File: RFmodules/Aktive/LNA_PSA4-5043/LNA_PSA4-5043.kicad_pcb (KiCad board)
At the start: 2 copper layers, 18 x 7.6 mm, 7 parts, among them U1 PSA4-5043+

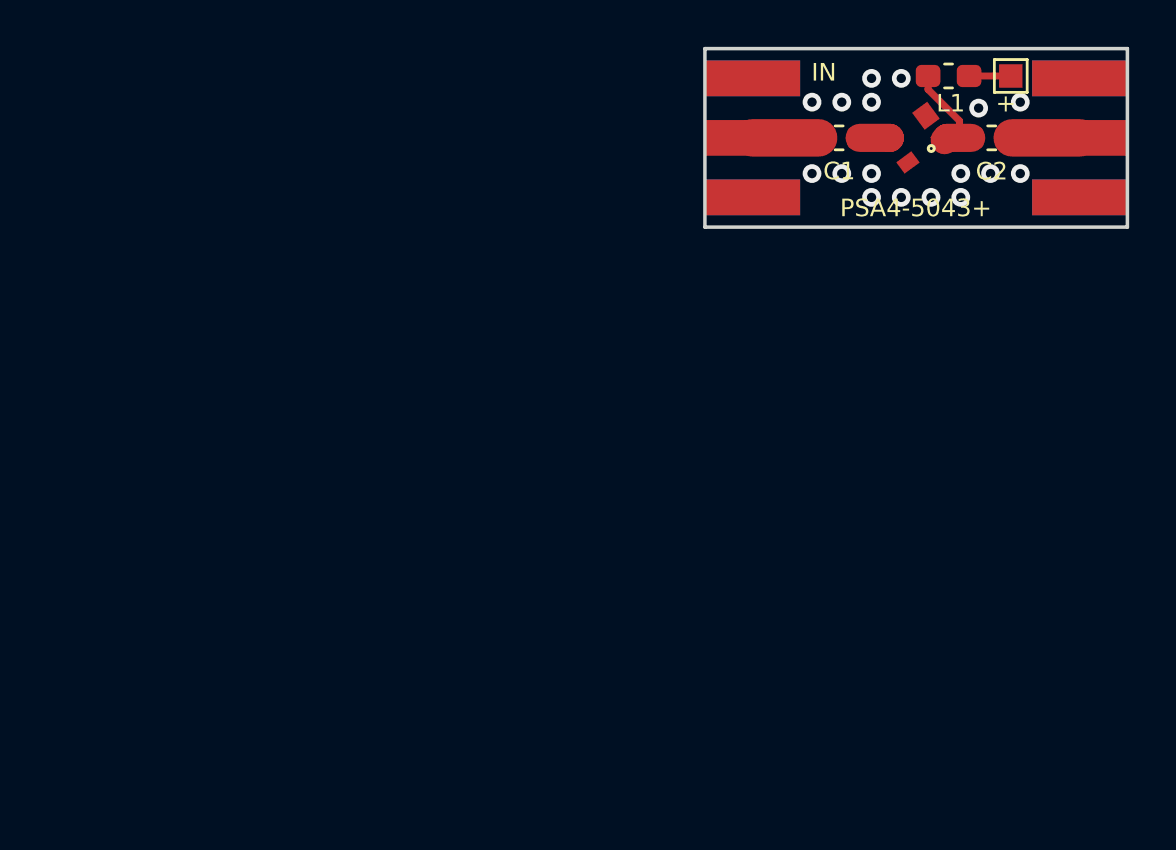
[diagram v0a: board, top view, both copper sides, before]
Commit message: Update LNA PSA4-5043 module to use new template
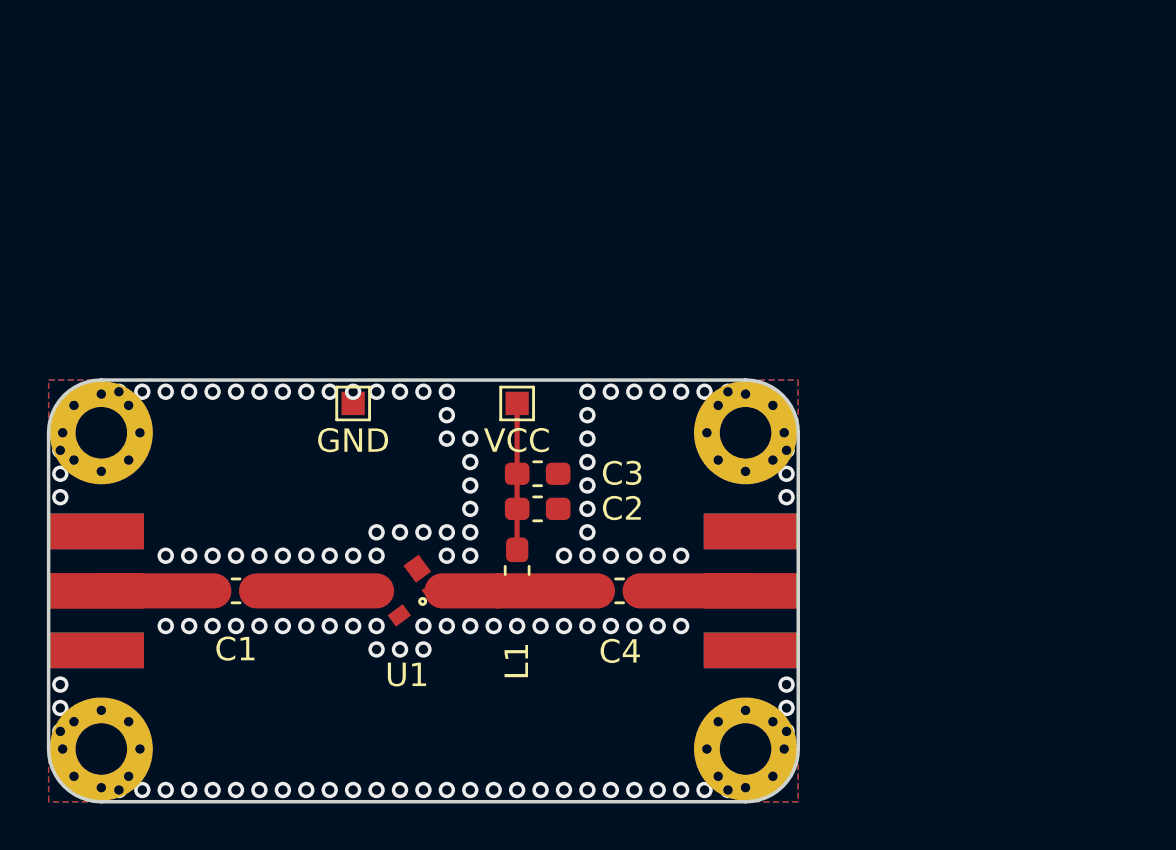
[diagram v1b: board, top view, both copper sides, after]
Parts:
- removed +: TestPoint, TestPoint:TestPoint_Pad_1.0x1.0mm
- removed IN, OUT: SMA, RFLego_Footprint:SMA_Edge
- added C3: C, Capacitor_SMD:C_0603_1608Metric_Pad1.05x0.95mm_HandSolder, F.Cu at (120.9, 104.0)
- added C4: C, Capacitor_SMD:C_0603_1608Metric_Pad1.05x0.95mm_HandSolder, F.Cu at (124.4, 109.0)
- added GND: GND, TestPoint:TestPoint_Pad_1.0x1.0mm, F.Cu at (113.0, 101.0)
- added H1: MountingHole_Pad, MountingHole:MountingHole_2.2mm_M2_Pad_Via, F.Cu at (102.2, 102.2)
- added H2: MountingHole_Pad, MountingHole:MountingHole_2.2mm_M2_Pad_Via, F.Cu at (102.2, 115.8)
- added H3: MountingHole_Pad, MountingHole:MountingHole_2.2mm_M2_Pad_Via, F.Cu at (129.8, 102.2)
- added H4: MountingHole_Pad, MountingHole:MountingHole_2.2mm_M2_Pad_Via, F.Cu at (129.8, 115.8)
- added J1: SMA, RFLego_Footprint:SMA_Edge, F.Cu at (100.0, 109.0)
- added J2: SMA, RFLego_Footprint:SMA_Edge, F.Cu at (128.0, 109.0)
- added REF**: OSHW-Logo2_9.8x8mm_SilkScreen, Symbol:OSHW-Logo2_9.8x8mm_SilkScreen, B.Cu at (109.5, 113.0)
- added VCC: VCC, TestPoint:TestPoint_Pad_1.0x1.0mm, F.Cu at (120.0, 101.0)
- C1, C2: value 10 nF -> C
- moved C1 32.2 mm to (108.0, 109.0)
- moved U1 29.1 mm to (115.3, 109.0)
- moved L1 28.0 mm to (120.0, 108.1), turned to 270 degrees
- moved C2 25.0 mm to (120.9, 105.5)
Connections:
- C2 pad 1: Net-(C2-Pad1) -> GND
- L1 pad 1: Net-(L1-Pad1) -> Net-(C2-Pad2)
- L1 pad 2: Net-(C2-Pad2) -> Net-(C4-Pad2)
- U1 pad 1: Net-(C2-Pad2) -> Net-(C4-Pad2)
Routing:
- net Net-(C4-Pad2): track 0.00 -> 6.37 mm
- net Net-(C4-Pad1): track 0.00 -> 4.75 mm
- net Net-(C1-Pad1): track 1.29 -> 5.13 mm
- net Net-(C2-Pad1): track 2.88 -> 0.00 mm
- net Net-(C1-Pad2): track 2.82 -> 5.02 mm
- net Net-(L1-Pad1): track 1.78 -> 0.00 mm
- net Net-(C2-Pad2): track 5.08 -> 6.25 mm
- net GND: vias 17 -> 121
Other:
- board size 18 x 7.6 mm -> 32 x 18 mm
- net class 0603 removed
- net class 50 Ohm thin added: clearance 0.19, trace_width 1, via_dia 0.7, via_drill 0.4
- net class 50Ohm added: clearance 0.32, trace_width 1.5, via_dia 0.7, via_drill 0.4
- net class Default: trace_width 0.3 -> 0.22; via_dia 0.8 -> 0.7
- net class RF removed
- rule via_min_size: 0.4 -> 0.6
- board text added: "PSA4-5043+ Revision 2 - 02/2019 github.com/fgaletsee/RFLego"
- board text removed: "LNA PSA4-5043+ Revision 1 - 01/2019 github.com/fgaletsee/RFLego"
